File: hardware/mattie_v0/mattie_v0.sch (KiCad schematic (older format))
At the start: 0 parts

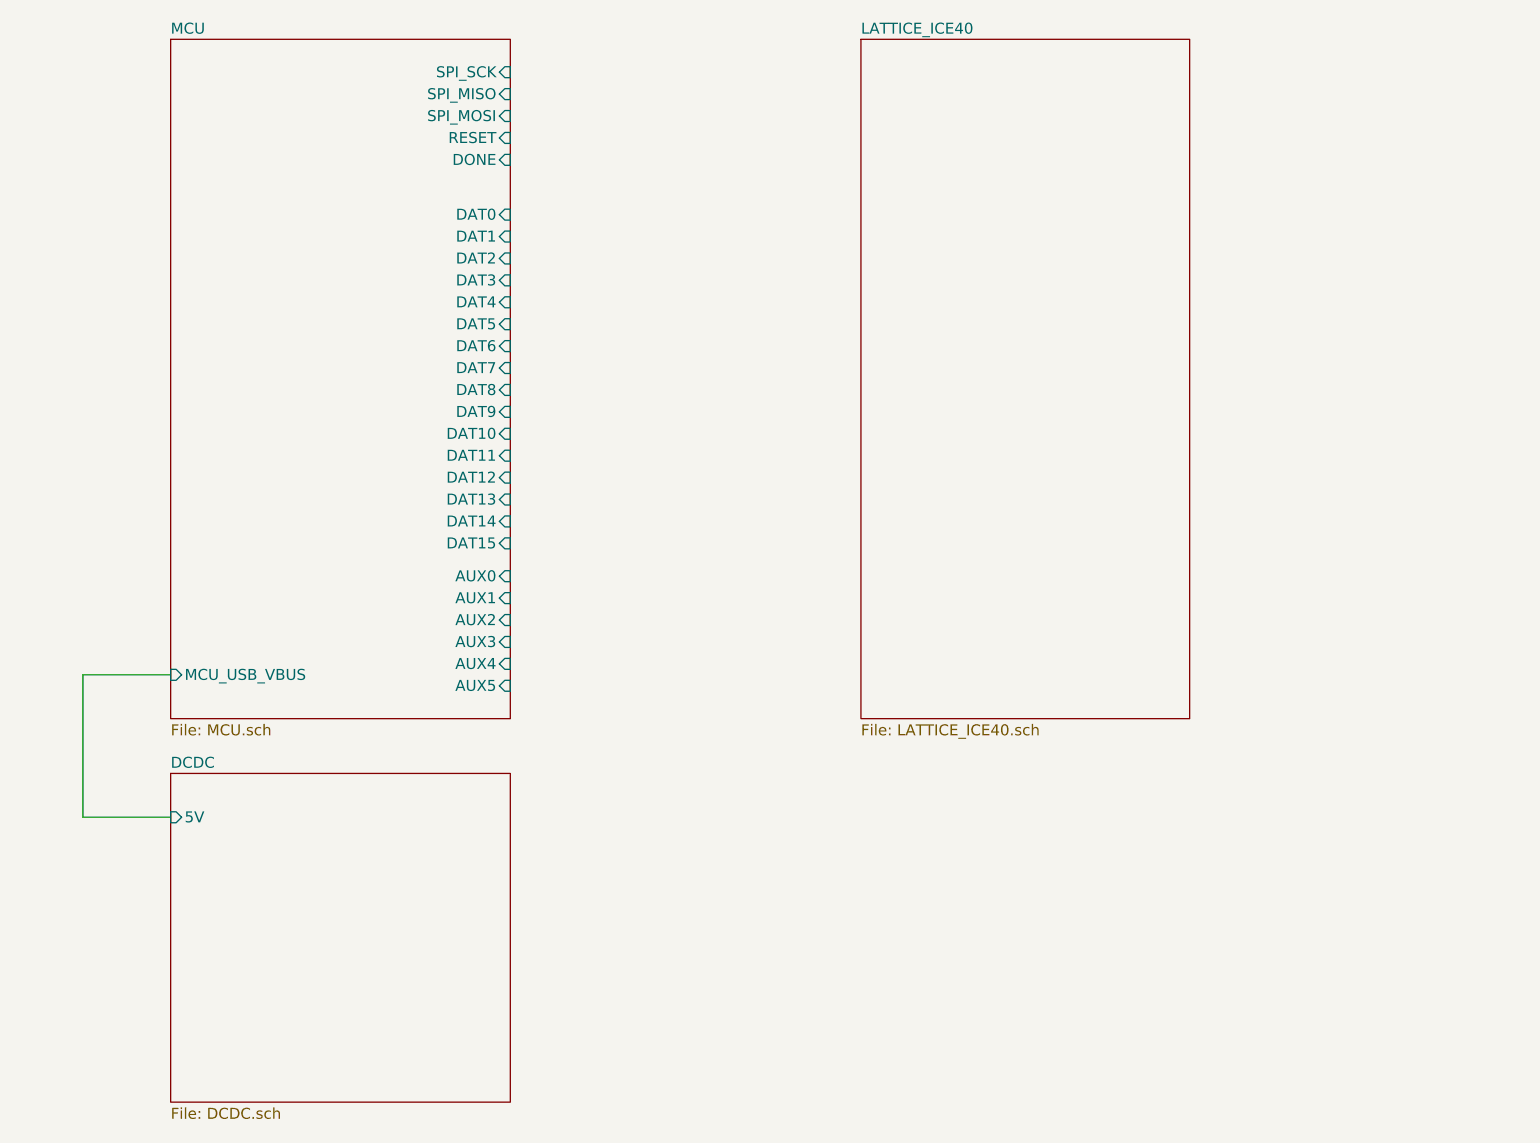
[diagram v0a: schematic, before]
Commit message: some tweaks
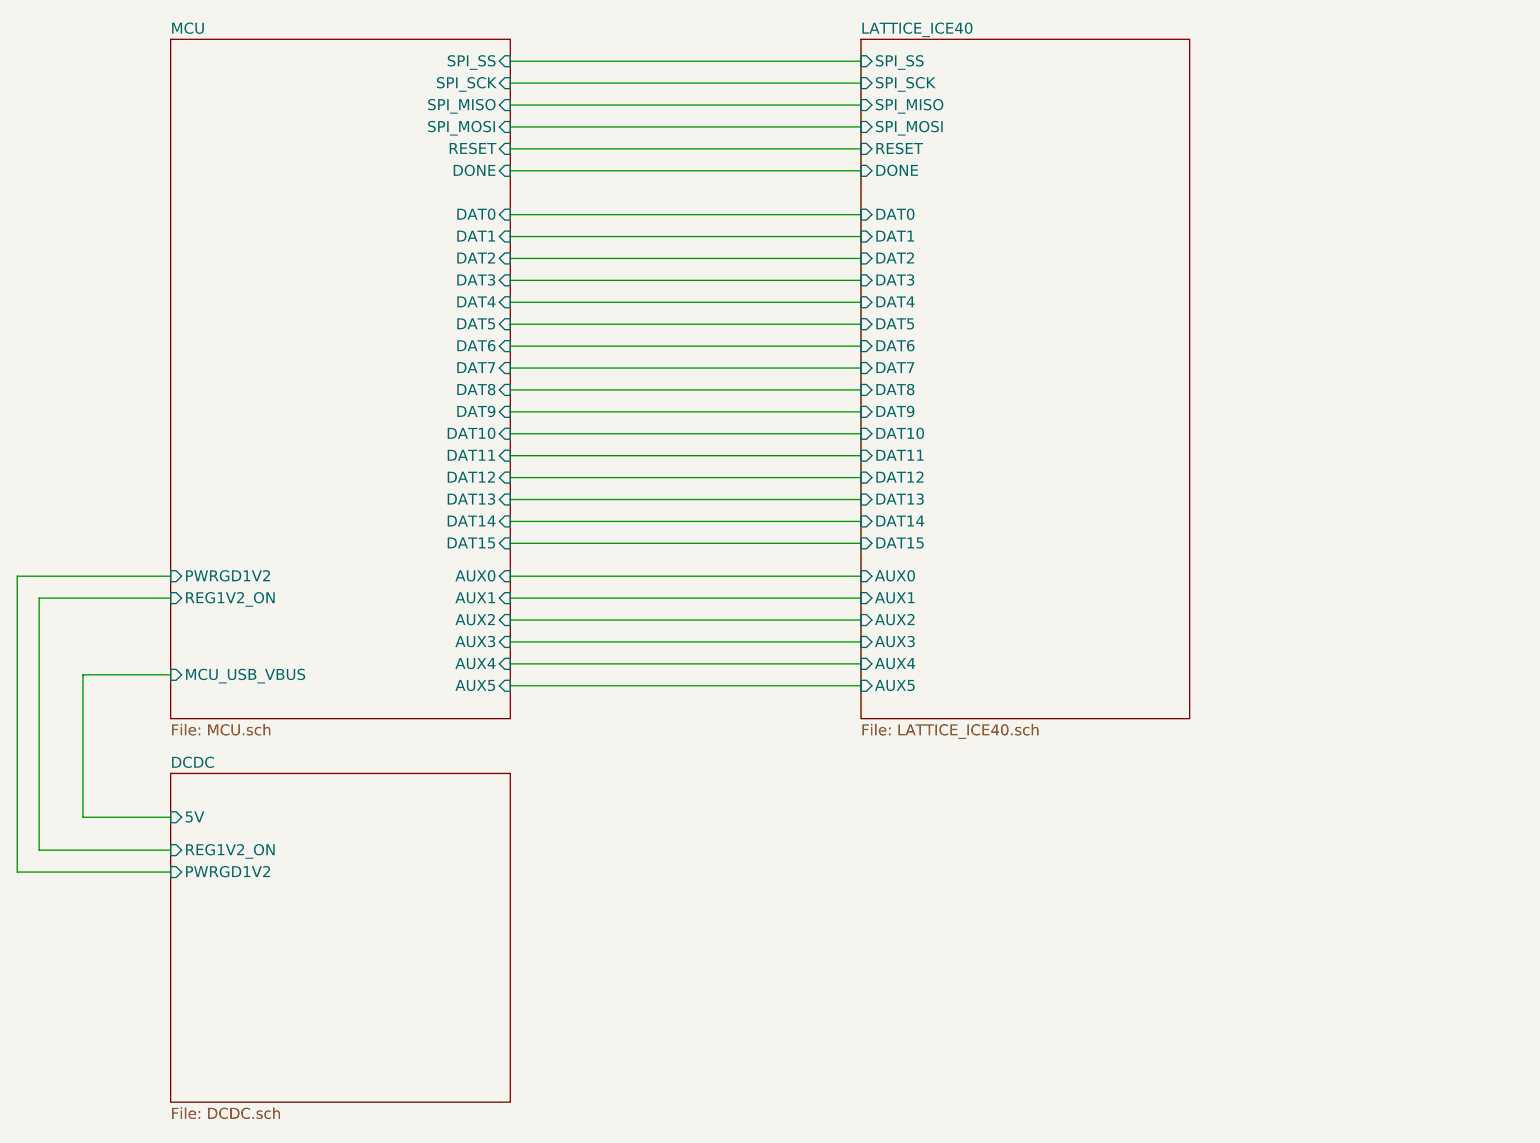
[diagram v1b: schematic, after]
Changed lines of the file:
@@
 F0 "MCU" 50
 F1 "MCU.sch" 50
-F2 "SPI_SCK" I R 3950 1150 50
-F3 "SPI_MISO" I R 3950 1250 50
-F4 "SPI_MOSI" I R 3950 1350 50
-F5 "RESET" I R 3950 1450 50
-F6 "DONE" I R 3950 1550 50
+F2 "SPI_SCK" I R 3950 1200 50
+F3 "SPI_MISO" I R 3950 1300 50
+F4 "SPI_MOSI" I R 3950 1400 50
+F5 "RESET" I R 3950 1500 50
+F6 "DONE" I R 3950 1600 50
 F7 "MCU_USB_VBUS" I L 2400 3900 50
 F8 "DAT0" I R 3950 1800 50
@@
 F28 "AUX4" I R 3950 3850 50
 F29 "AUX5" I R 3950 3950 50
+F30 "REG1V2_ON" I L 2400 3550 50
+F31 "PWRGD1V2" I L 2400 3450 50
+F32 "SPI_SS" I R 3950 1100 50
 $EndSheet
 $Sheet
@@
 F1 "DCDC.sch" 50
 F2 "5V" I L 2400 4550 50
+F3 "REG1V2_ON" I L 2400 4700 50
+F4 "PWRGD1V2" I L 2400 4800 50
 $EndSheet
 $Sheet
@@
 F0 "LATTICE_ICE40" 50
 F1 "LATTICE_ICE40.sch" 50
+F2 "SPI_SS" I L 5550 1100 50
+F3 "SPI_SCK" I L 5550 1200 50
+F4 "SPI_MISO" I L 5550 1300 50
+F5 "SPI_MOSI" I L 5550 1400 50
+F6 "RESET" I L 5550 1500 50
+F7 "DONE" I L 5550 1600 50
+F8 "DAT0" I L 5550 1800 50
+F9 "DAT1" I L 5550 1900 50
+F10 "DAT2" I L 5550 2000 50
+F11 "DAT3" I L 5550 2100 50
+F12 "DAT4" I L 5550 2200 50
+F13 "DAT5" I L 5550 2300 50
+F14 "DAT6" I L 5550 2400 50
+F15 "DAT7" I L 5550 2500 50
+F16 "DAT8" I L 5550 2600 50
+F17 "DAT9" I L 5550 2700 50
+F18 "DAT10" I L 5550 2800 50
+F19 "DAT11" I L 5550 2900 50
+F20 "DAT12" I L 5550 3000 50
+F21 "DAT13" I L 5550 3100 50
+F22 "DAT14" I L 5550 3200 50
+F23 "DAT15" I L 5550 3300 50
+F24 "AUX0" I L 5550 3450 50
+F25 "AUX1" I L 5550 3550 50
+F26 "AUX2" I L 5550 3650 50
+F27 "AUX3" I L 5550 3750 50
+F28 "AUX4" I L 5550 3850 50
+F29 "AUX5" I L 5550 3950 50
 $EndSheet
 Wire Wire Line
@@
 Wire Wire Line
 	2000 4550 2400 4550
+Wire Wire Line
+	2400 4700 1800 4700
+Wire Wire Line
+	1800 4700 1800 3550
+Wire Wire Line
+	1800 3550 2400 3550
+Wire Wire Line
+	2400 3450 1700 3450
+Wire Wire Line
+	1700 3450 1700 4800
+Wire Wire Line
+	1700 4800 2400 4800
+Wire Wire Line
+	3950 1100 5550 1100
+Wire Wire Line
+	3950 1200 5550 1200
+Wire Wire Line
+	3950 1300 5550 1300
+Wire Wire Line
+	3950 1400 5550 1400
+Wire Wire Line
+	3950 1500 5550 1500
+Wire Wire Line
+	3950 1600 5550 1600
+Wire Wire Line
+	5550 3300 3950 3300
+Wire Wire Line
+	3950 3200 5550 3200
+Wire Wire Line
+	5550 3100 3950 3100
+Wire Wire Line
+	3950 3000 5550 3000
+Wire Wire Line
+	5550 2900 3950 2900
+Wire Wire Line
+	3950 2800 5550 2800
+Wire Wire Line
+	5550 2700 3950 2700
+Wire Wire Line
+	3950 2600 5550 2600
+Wire Wire Line
+	5550 2500 3950 2500
+Wire Wire Line
+	3950 2400 5550 2400
+Wire Wire Line
+	5550 2300 3950 2300
+Wire Wire Line
+	3950 2200 5550 2200
+Wire Wire Line
+	5550 2100 3950 2100
+Wire Wire Line
+	3950 2000 5550 2000
+Wire Wire Line
+	5550 1900 3950 1900
+Wire Wire Line
+	3950 1800 5550 1800
+Wire Wire Line
+	3950 3450 5550 3450
+Wire Wire Line
+	5550 3550 3950 3550
+Wire Wire Line
+	3950 3650 5550 3650
+Wire Wire Line
+	5550 3750 3950 3750
+Wire Wire Line
+	3950 3850 5550 3850
+Wire Wire Line
+	5550 3950 3950 3950
 $EndSCHEMATC

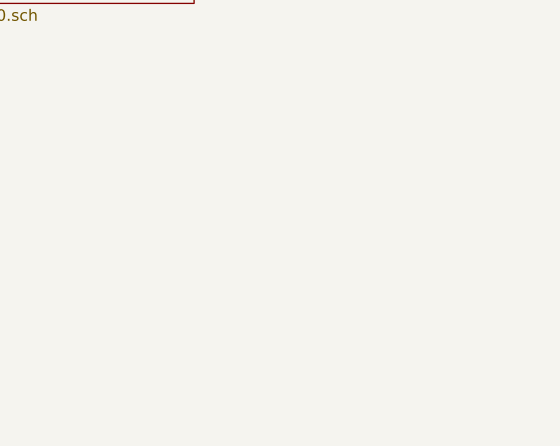
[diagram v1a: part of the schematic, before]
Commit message: update
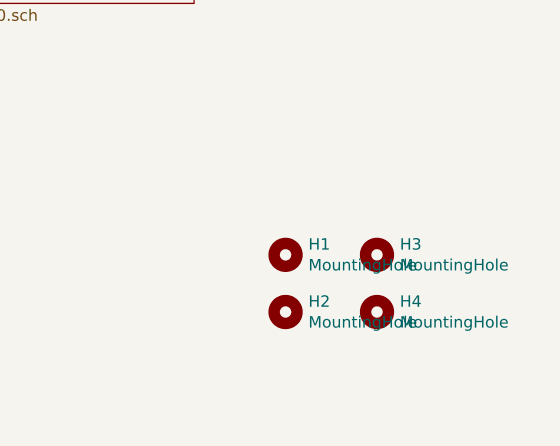
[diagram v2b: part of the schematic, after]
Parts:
- added H1, H2, H3, H4: MountingHole, MountingHole:MountingHole_3.2mm_M3, symbol Mechanical:MountingHole
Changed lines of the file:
@@
 Wire Wire Line
 	5550 3950 3950 3950
+$Comp
+L Mechanical:MountingHole H3
+U 1 1 5EA5CE8F
+P 7850 5200
+F 0 "H3" H 7950 5246 50  0000 L CNN
+F 1 "MountingHole" H 7950 5155 50  0000 L CNN
+F 2 "MountingHole:MountingHole_3.2mm_M3" H 7850 5200 50  0001 C CNN
+F 3 "~" H 7850 5200 50  0001 C CNN
+	1    7850 5200
+	1    0    0    -1
+$EndComp
+$Comp
+L Mechanical:MountingHole H1
+U 1 1 5EA5CF8D
+P 7450 5200
+F 0 "H1" H 7550 5246 50  0000 L CNN
+F 1 "MountingHole" H 7550 5155 50  0000 L CNN
+F 2 "MountingHole:MountingHole_3.2mm_M3" H 7450 5200 50  0001 C CNN
+F 3 "~" H 7450 5200 50  0001 C CNN
+	1    7450 5200
+	1    0    0    -1
+$EndComp
+$Comp
+L Mechanical:MountingHole H2
+U 1 1 5EA5D0B7
+P 7450 5450
+F 0 "H2" H 7550 5496 50  0000 L CNN
+F 1 "MountingHole" H 7550 5405 50  0000 L CNN
+F 2 "MountingHole:MountingHole_3.2mm_M3" H 7450 5450 50  0001 C CNN
+F 3 "~" H 7450 5450 50  0001 C CNN
+	1    7450 5450
+	1    0    0    -1
+$EndComp
+$Comp
+L Mechanical:MountingHole H4
+U 1 1 5EA5D2F7
+P 7850 5450
+F 0 "H4" H 7950 5496 50  0000 L CNN
+F 1 "MountingHole" H 7950 5405 50  0000 L CNN
+F 2 "MountingHole:MountingHole_3.2mm_M3" H 7850 5450 50  0001 C CNN
+F 3 "~" H 7850 5450 50  0001 C CNN
+	1    7850 5450
+	1    0    0    -1
+$EndComp
 $EndSCHEMATC
